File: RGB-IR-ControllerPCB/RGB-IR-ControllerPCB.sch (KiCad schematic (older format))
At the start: 16 parts, among them J1 Conn_01x02_Female, J2 Conn_01x01_Female, J3 Conn_01x01_Female, J4 Conn_01x01_Female, J5 Conn_01x01_Female, Q1 IRF540N, Q2 IRF540N, Q3 IRF540N, U1 TSOP17xx

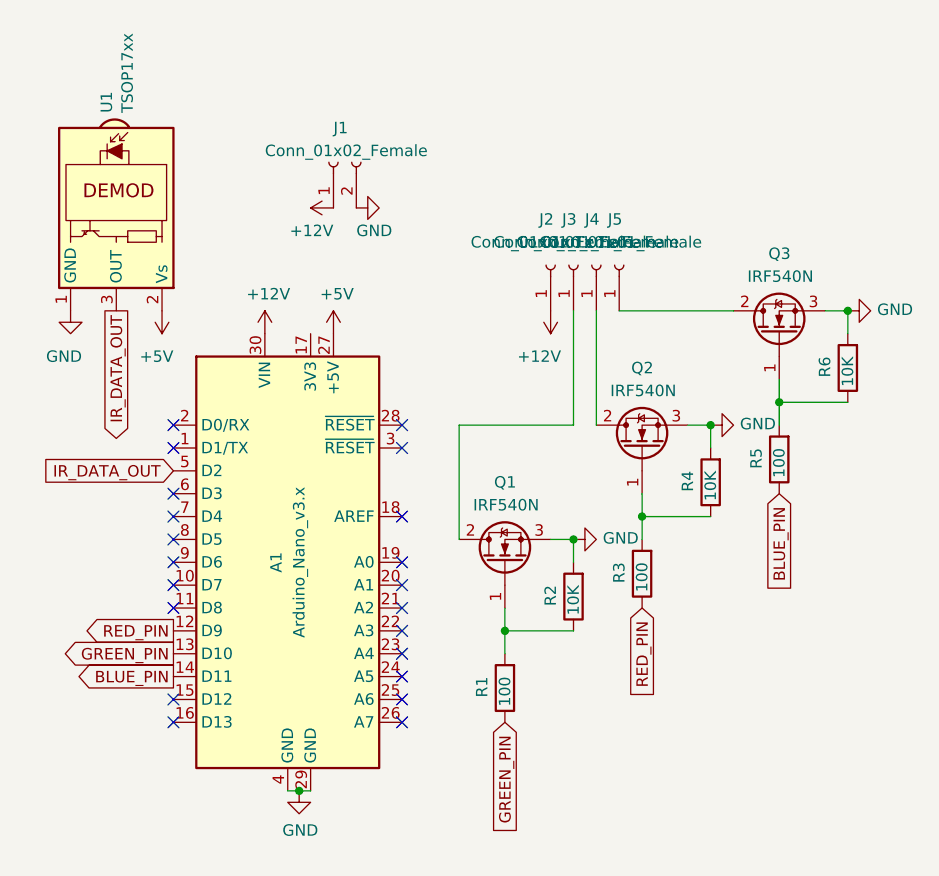
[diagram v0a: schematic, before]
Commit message: Updated PCB and clear deprecate code
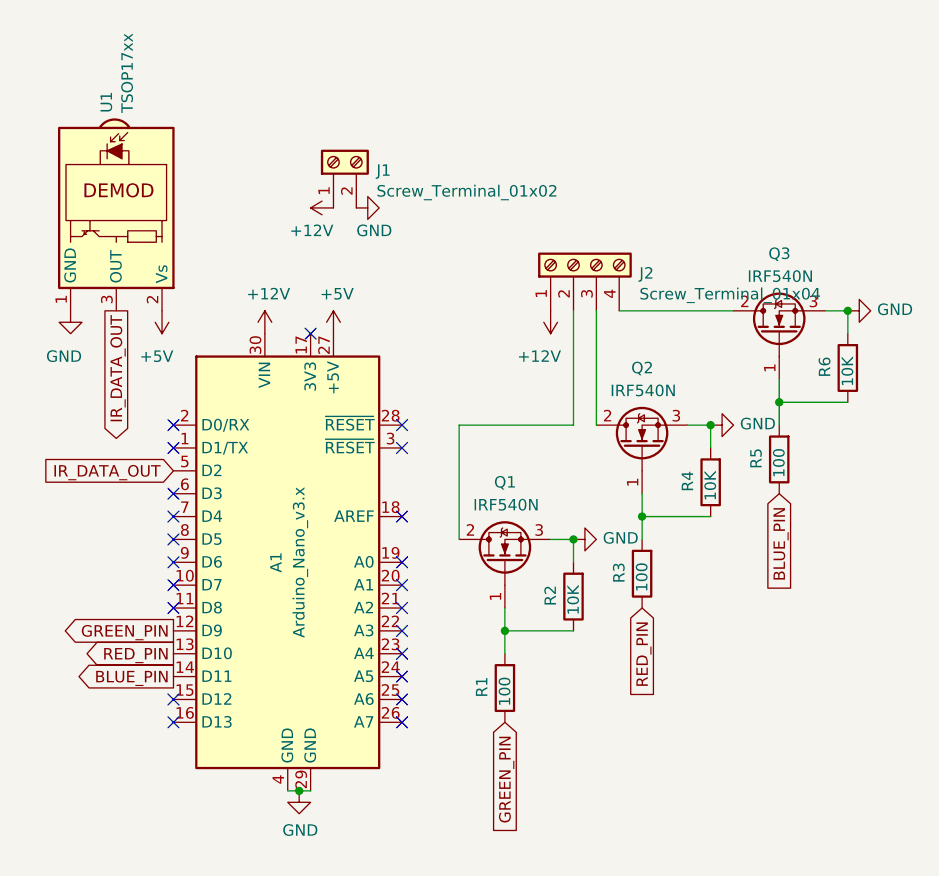
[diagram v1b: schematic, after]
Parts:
- removed J1: Conn_01x02_Female, TerminalBlock:TerminalBlock_bornier-2_P5.08mm, symbol Connector:Conn_01x02_Female
- removed J2, J3, J4, J5: Conn_01x01_Female, Connector_Pin:Pin_D1.4mm_L8.5mm_W2.8mm_FlatFork, symbol Connector:Conn_01x01_Female
- added J1: Screw_Terminal_01x02, TerminalBlock:TerminalBlock_Altech_AK300-2_P5.00mm, symbol Connector:Screw_Terminal_01x02
- added J2: Screw_Terminal_01x04, TerminalBlock:TerminalBlock_Altech_AK300-4_P5.00mm, symbol Connector:Screw_Terminal_01x04
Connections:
- net +12V: now also J1.1 (Pin_1), J2.1 (Pin_1)
- net GND: now also J1.2 (Pin_2)
- net GREEN_PIN: now also A1.12 (D9); no longer A1.13 (D10)
- net RED_PIN: now also A1.13 (D10); no longer A1.12 (D9)
- net at Q2.2 (D): now also J2.3 (Pin_3)
- net at Q1.2 (D): now also J2.2 (Pin_2)
- net at Q3.2 (D): now also J2.4 (Pin_4)
- no-connect marks 21 -> 22
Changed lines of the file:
@@
 $EndComp
 $Comp
-L power:GND #PWR0101
+L power:GND #PWR04
 U 1 1 606A1DF2
 P 1600 7550
-F 0 "#PWR0101" H 1600 7300 50  0001 C CNN
+F 0 "#PWR04" H 1600 7300 50  0001 C CNN
 F 1 "GND" H 1605 7377 50  0000 C CNN
 F 2 "" H 1600 7550 50  0001 C CNN
@@
 	1600 7550 1550 7550
 $Comp
-L power:GND #PWR0102
+L power:GND #PWR01
 U 1 1 606A7797
 P 600 5450
-F 0 "#PWR0102" H 600 5200 50  0001 C CNN
+F 0 "#PWR01" H 600 5200 50  0001 C CNN
 F 1 "GND" H 650 5250 50  0000 R CNN
 F 2 "" H 600 5450 50  0001 C CNN
@@
 $EndComp
 $Comp
-L power:+12V #PWR0103
+L power:+12V #PWR03
 U 1 1 606A8AEB
 P 1450 5550
-F 0 "#PWR0103" H 1450 5400 50  0001 C CNN
+F 0 "#PWR03" H 1450 5400 50  0001 C CNN
 F 1 "+12V" H 1465 5723 50  0000 C CNN
 F 2 "" H 1450 5550 50  0001 C CNN
@@
 $EndComp
 $Comp
-L power:+5V #PWR0104
+L power:+5V #PWR06
 U 1 1 606A9E07
 P 1750 5550
-F 0 "#PWR0104" H 1750 5400 50  0001 C CNN
+F 0 "#PWR06" H 1750 5400 50  0001 C CNN
 F 1 "+5V" H 1765 5723 50  0000 C CNN
 F 2 "" H 1750 5550 50  0001 C CNN
@@
 $EndComp
 $Comp
-L power:+5V #PWR0105
+L power:+5V #PWR02
 U 1 1 606AA3ED
 P 1000 5450
-F 0 "#PWR0105" H 1000 5300 50  0001 C CNN
+F 0 "#PWR02" H 1000 5300 50  0001 C CNN
 F 1 "+5V" H 950 5650 50  0000 L CNN
 F 2 "" H 1000 5450 50  0001 C CNN
@@
 	1    0    0    -1
 $EndComp
+Text GLabel 1050 6950 0    50   Output ~ 0
+RED_PIN
 Text GLabel 1050 6850 0    50   Output ~ 0
-RED_PIN
-Text GLabel 1050 6950 0    50   Output ~ 0
 GREEN_PIN
 Text GLabel 1050 7050 0    50   Output ~ 0
@@
 	2800 6450 2700 6450
 $Comp
-L power:GND #PWR0106
+L power:GND #PWR010
 U 1 1 6078840F
 P 3400 5950
-F 0 "#PWR0106" H 3400 5700 50  0001 C CNN
+F 0 "#PWR010" H 3400 5700 50  0001 C CNN
 F 1 "GND" V 3405 5822 50  0000 R CNN
 F 2 "" H 3400 5950 50  0001 C CNN
@@
 $EndComp
 $Comp
-L power:GND #PWR0107
+L power:GND #PWR09
 U 1 1 6078955C
 P 2800 6450
-F 0 "#PWR0107" H 2800 6200 50  0001 C CNN
+F 0 "#PWR09" H 2800 6200 50  0001 C CNN
 F 1 "GND" V 2805 6322 50  0000 R CNN
 F 2 "" H 2800 6450 50  0001 C CNN
@@
 	4000 5550 4000 5450
 $Comp
-L power:GND #PWR0108
+L power:GND #PWR011
 U 1 1 60789AFF
 P 4000 5450
-F 0 "#PWR0108" H 4000 5200 50  0001 C CNN
+F 0 "#PWR011" H 4000 5200 50  0001 C CNN
 F 1 "GND" V 4005 5322 50  0000 R CNN
 F 2 "" H 4000 5450 50  0001 C CNN
@@
 $EndComp
 $Comp
-L power:+12V #PWR0109
+L power:+12V #PWR08
 U 1 1 6080C130
 P 2700 5450
-F 0 "#PWR0109" H 2700 5300 50  0001 C CNN
+F 0 "#PWR08" H 2700 5300 50  0001 C CNN
 F 1 "+12V" H 2750 5650 50  0000 C CNN
 F 2 "" H 2700 5450 50  0001 C CNN
@@
 $EndComp
 $Comp
-L Connector:Conn_01x02_Female J1
-U 1 1 60874EB8
-P 1750 4800
-F 0 "J1" V 1900 4800 50  0000 R CNN
-F 1 "Conn_01x02_Female" V 1800 5100 50  0000 R CNN
-F 2 "TerminalBlock:TerminalBlock_bornier-2_P5.08mm" H 1750 4800 50  0001 C CNN
-F 3 "~" H 1750 4800 50  0001 C CNN
-	1    1750 4800
-	0    -1   -1   0
-$EndComp
-$Comp
-L power:+12V #PWR0110
+L power:+12V #PWR05
 U 1 1 6087ADC9
 P 1750 5000
-F 0 "#PWR0110" H 1750 4850 50  0001 C CNN
+F 0 "#PWR05" H 1750 4850 50  0001 C CNN
 F 1 "+12V" V 1650 5000 50  0000 L CNN
 F 2 "" H 1750 5000 50  0001 C CNN
@@
 $EndComp
 $Comp
-L power:GND #PWR0111
+L power:GND #PWR07
 U 1 1 6087B56C
 P 1850 5000
-F 0 "#PWR0111" H 1850 4750 50  0001 C CNN
+F 0 "#PWR07" H 1850 4750 50  0001 C CNN
 F 1 "GND" V 1750 5000 50  0000 R CNN
 F 2 "" H 1850 5000 50  0001 C CNN
@@
 $EndComp
 $Comp
-L Connector:Conn_01x01_Female J2
-U 1 1 608A8D29
-P 2700 5250
-F 0 "J2" V 2900 5300 50  0000 R CNN
-F 1 "Conn_01x01_Female" V 2800 5600 50  0000 R CNN
-F 2 "Connector_Pin:Pin_D1.4mm_L8.5mm_W2.8mm_FlatFork" H 2700 5250 50  0001 C CNN
-F 3 "~" H 2700 5250 50  0001 C CNN
-	1    2700 5250
-	0    -1   -1   0
-$EndComp
-$Comp
-L Connector:Conn_01x01_Female J3
-U 1 1 608AA3D2
+L Connector:Screw_Terminal_01x04 J2
+U 1 1 606ECFF6
 P 2800 5250
-F 0 "J3" V 3000 5300 50  0000 R CNN
-F 1 "Conn_01x01_Female" V 2900 5600 50  0000 R CNN
-F 2 "Connector_Pin:Pin_D1.4mm_L8.5mm_W2.8mm_FlatFork" H 2800 5250 50  0001 C CNN
+F 0 "J2" V 2764 4962 50  0000 R CNN
+F 1 "Screw_Terminal_01x04" V 2673 4962 50  0000 R CNN
+F 2 "TerminalBlock:TerminalBlock_Altech_AK300-4_P5.00mm" H 2800 5250 50  0001 C CNN
 F 3 "~" H 2800 5250 50  0001 C CNN
 	1    2800 5250
@@
 $EndComp
 $Comp
-L Connector:Conn_01x01_Female J4
-U 1 1 608AA967
-P 2900 5250
-F 0 "J4" V 3100 5300 50  0000 R CNN
-F 1 "Conn_01x01_Female" V 3000 5600 50  0000 R CNN
-F 2 "Connector_Pin:Pin_D1.4mm_L8.5mm_W2.8mm_FlatFork" H 2900 5250 50  0001 C CNN
-F 3 "~" H 2900 5250 50  0001 C CNN
-	1    2900 5250
-	0    -1   -1   0
-$EndComp
-$Comp
-L Connector:Conn_01x01_Female J5
-U 1 1 608AAF24
-P 3000 5250
-F 0 "J5" V 3200 5300 50  0000 R CNN
-F 1 "Conn_01x01_Female" V 3100 5600 50  0000 R CNN
-F 2 "Connector_Pin:Pin_D1.4mm_L8.5mm_W2.8mm_FlatFork" H 3000 5250 50  0001 C CNN
-F 3 "~" H 3000 5250 50  0001 C CNN
-	1    3000 5250
-	0    -1   -1   0
-$EndComp
+L Connector:Screw_Terminal_01x02 J1
+U 1 1 606EE485
+P 1750 4800
+F 0 "J1" V 1714 4612 50  0000 R CNN
+F 1 "Screw_Terminal_01x02" V 1623 4612 50  0000 R CNN
+F 2 "TerminalBlock:TerminalBlock_Altech_AK300-2_P5.00mm" H 1750 4800 50  0001 C CNN
+F 3 "~" H 1750 4800 50  0001 C CNN
+	1    1750 4800
+	0    -1   -1   0
+$EndComp
+NoConn ~ 1650 5550
 $EndSCHEMATC

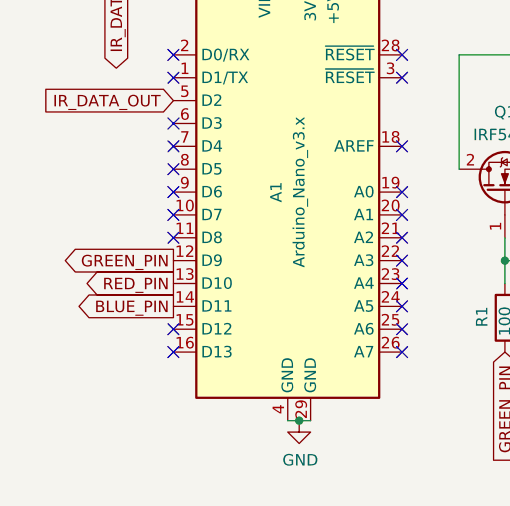
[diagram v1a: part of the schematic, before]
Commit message: Refactored PCB
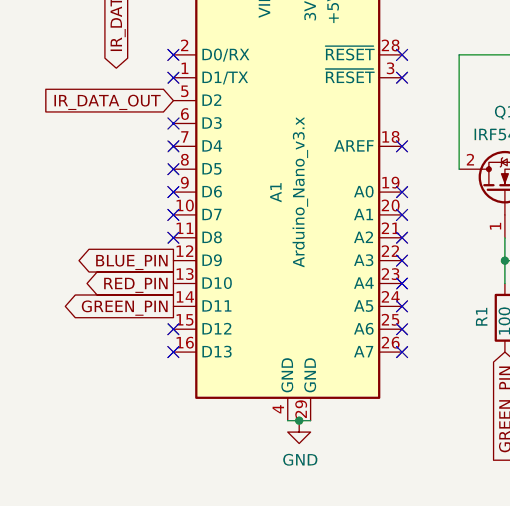
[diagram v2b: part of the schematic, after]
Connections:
- net BLUE_PIN: now also A1.12 (D9); no longer A1.14 (D11)
- net GREEN_PIN: now also A1.14 (D11); no longer A1.12 (D9)
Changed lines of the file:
@@
 Text GLabel 1050 6950 0    50   Output ~ 0
 RED_PIN
+Text GLabel 1050 7050 0    50   Output ~ 0
+GREEN_PIN
 Text GLabel 1050 6850 0    50   Output ~ 0
-GREEN_PIN
-Text GLabel 1050 7050 0    50   Output ~ 0
 BLUE_PIN
 Text GLabel 2500 7250 3    50   Input ~ 0
